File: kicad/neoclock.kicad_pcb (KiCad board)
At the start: 2 copper layers, 41.1 x 42.2 mm, 19 parts, among them CON1 2.1mm 5V, IC1 ATMEGA328P-A, K1 NEOPIXEL, P1 ICSP, P2 FTDI, SW1 HOUR, SW2 MINUTE, U1 DS1307

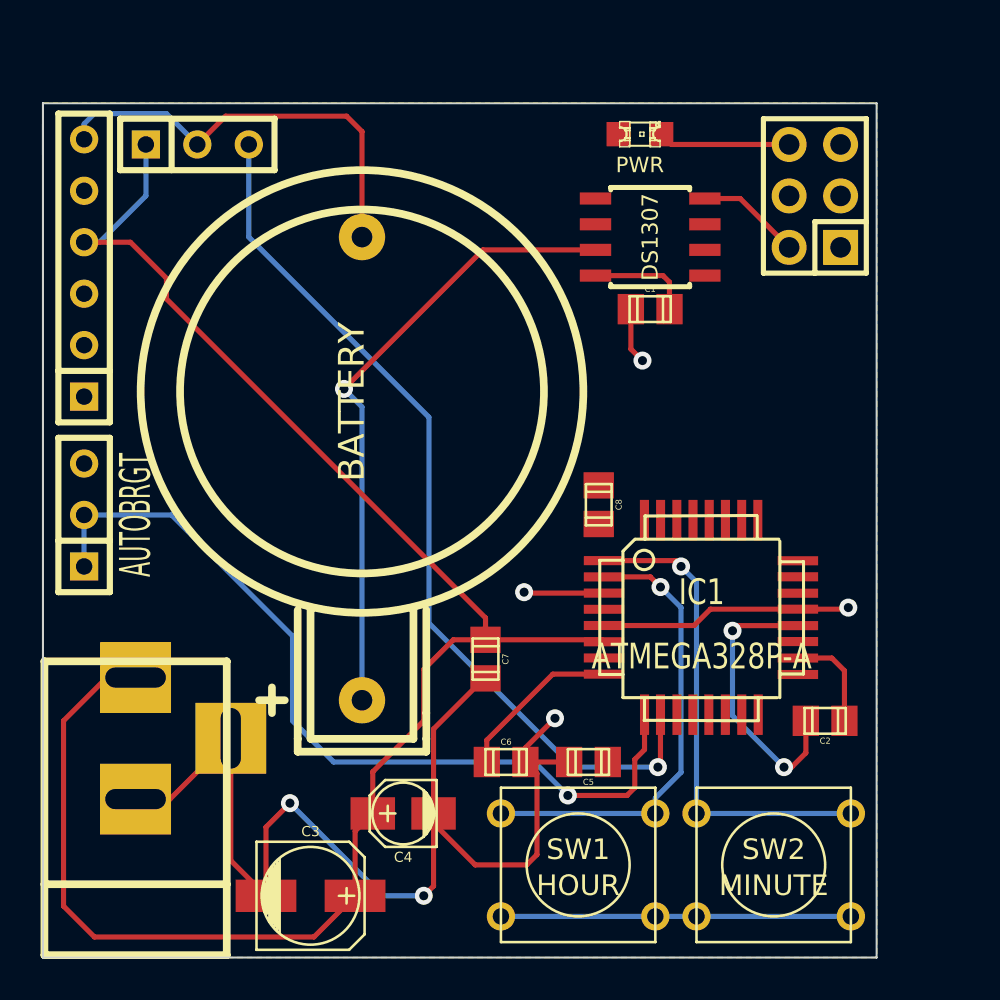
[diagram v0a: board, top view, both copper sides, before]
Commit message: woot
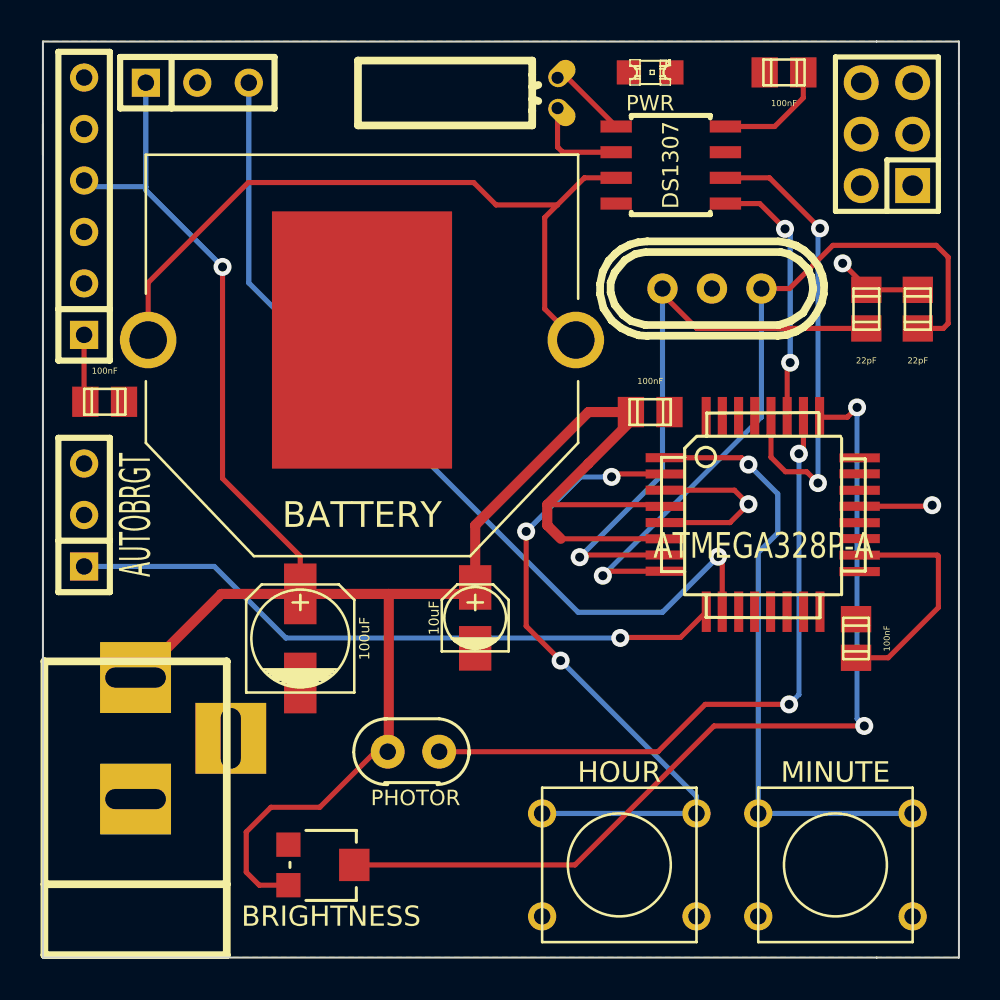
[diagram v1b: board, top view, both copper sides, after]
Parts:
- added PHOTOR1: PHOTOR, synic:PHOTORESISTOR, F.Cu at (114.8, 50.8)
- added RV1: BRIGHTNESS, synic:Timmer_Pot_ST32ETA103, F.Cu at (110.2, 56.4)
- added X1: 16Mhz, Crystals:Crystal_HC49-U_Vertical_3Pin, F.Cu at (129.5, 27.9)
- added X2: 32.768kHz, Crystals:Crystal_Round_Horizontal_3mm_BigPad, F.Cu at (121.9, 18.3)
- BT1: footprint Discret:CR2032H -> WANDL:WNL_CR2302_TH_KEYSTONE_3003
- moved C6 30.2 mm to (139.7, 29.0), turned to 90 degrees
- moved C5 26.2 mm to (137.2, 29.0), turned to 90 degrees
- moved C8 24.9 mm to (99.6, 33.5), turned to 180 degrees
- moved C7 14.7 mm to (126.5, 34.0), turned to 0 degrees
- moved C1 13.4 mm to (133.1, 17.3), turned to 180 degrees
- moved C3 12.7 mm to (109.2, 45.2), turned to 90 degrees
- moved C4 10.3 mm to (117.9, 44.2), turned to 90 degrees
- moved IC1 5.92 mm to (132.1, 39.1)
- moved P1 4.68 mm to (138.2, 20.3)
- moved C2 4.34 mm to (136.7, 45.2), turned to 90 degrees
- moved U1 3.70 mm to (127.5, 21.8)
- moved D1 3.09 mm to (126.5, 17.3)
- moved SW2 3.05 mm to (135.6, 56.4)
- moved K1 3.05 mm to (104.1, 17.8)
- moved P2 3.05 mm to (98.6, 23.9)
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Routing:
- net GND: track 123.1 -> 16.8 mm, vias 5 -> 3
- net BRIGHTNESS: track 0.00 -> 45.9 mm, vias 0 -> 2
- net Net-(IC1-Pad26): track 0.00 -> 32.7 mm, vias 0 -> 2
- net Net-(C5-Pad2): track 0.00 -> 30.3 mm, vias 0 -> 1
- net Net-(C6-Pad2): track 8.22 -> 35.8 mm, vias 0 -> 1
- net I2CSCL: track 0.00 -> 23.1 mm, vias 0 -> 2
- net VCC: track 100.4 -> 121.0 mm
- net Net-(C2-Pad1): track 14.1 -> 0.00 mm, vias 2 -> 0
- net I2CSDA: track 0.00 -> 12.9 mm, vias 0 -> 2
- net Net-(IC1-Pad2): track 22.7 -> 33.1 mm, vias 1 -> 3
- net Net-(IC1-Pad9): track 41.9 -> 32.7 mm
- net Net-(IC1-Pad1): track 24.0 -> 30.1 mm
- net Net-(BT1-Pad1): track 31.0 -> 36.5 mm, vias 1 -> 0
- net Net-(U1-Pad2): track 0.00 -> 4.91 mm
- net Net-(U1-Pad1): track 0.00 -> 3.89 mm
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- added copper zone on F.Cu, net GND
- removed copper zone on F.Cu, net VCC
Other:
- board size 41.1 x 42.2 mm -> 45.2 x 45.2 mm
